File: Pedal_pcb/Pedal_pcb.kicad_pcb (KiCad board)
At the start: 2 copper layers, 40.5 x 48.5 mm, 18 parts, among them U1 TL082

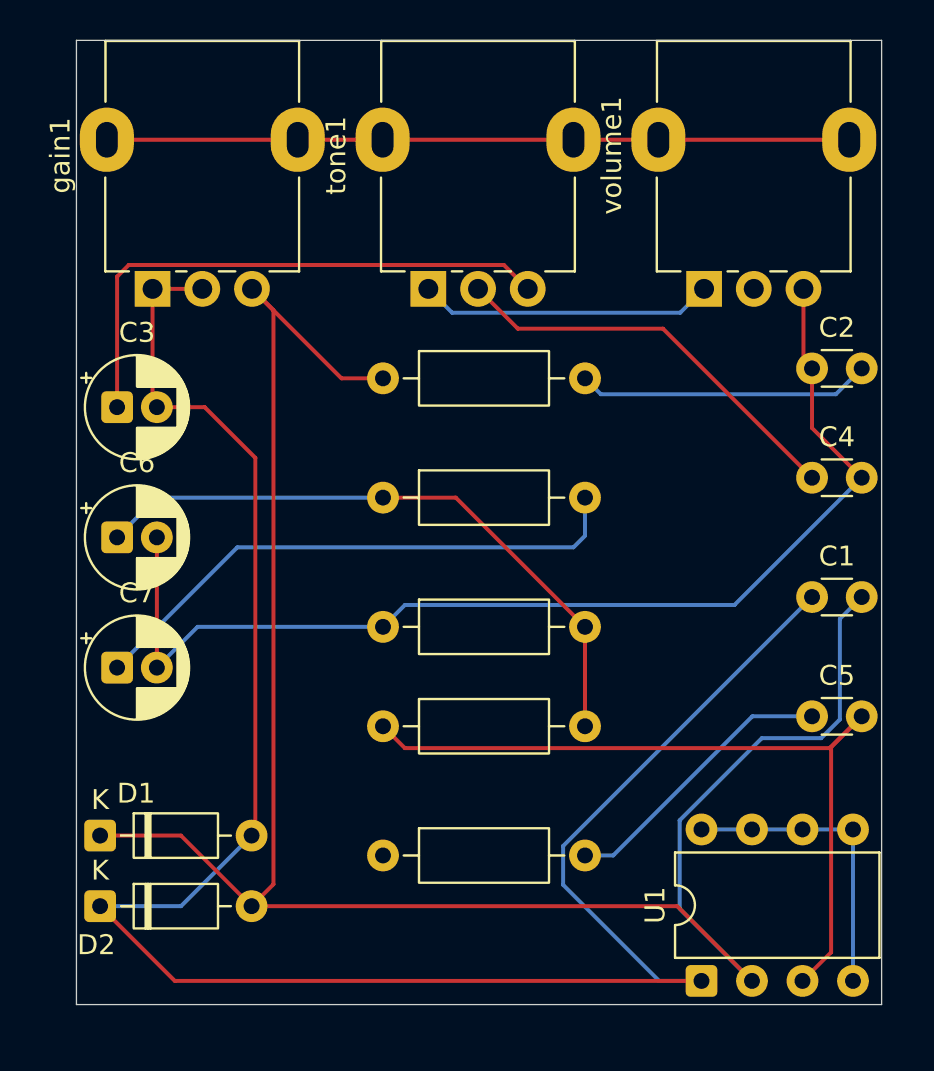
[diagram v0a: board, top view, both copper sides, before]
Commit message: better pcb design
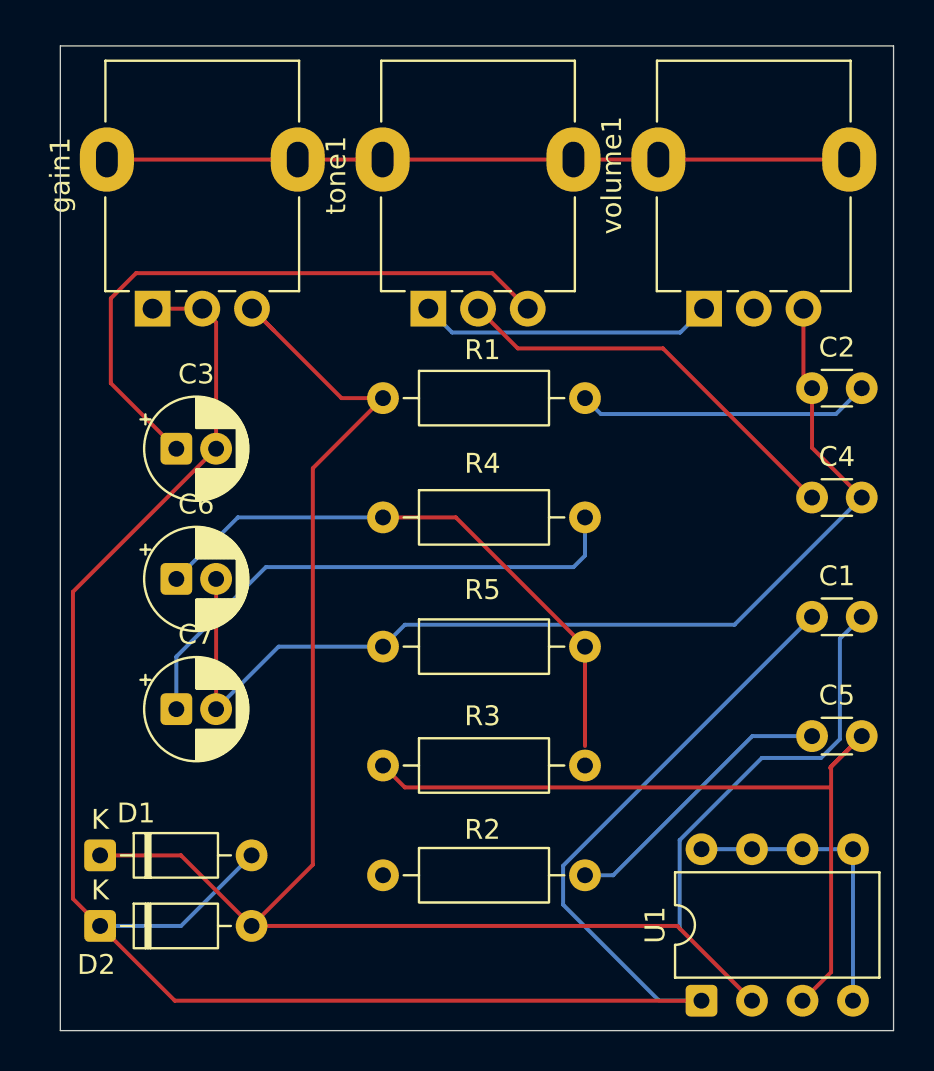
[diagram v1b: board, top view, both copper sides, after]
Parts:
- moved C6 3.64 mm to (129.0, 44.6)
- moved C7 3.64 mm to (129.0, 51.1)
- moved C3 3.64 mm to (129.0, 38.0)
- moved R3 1.98 mm to (139.4, 54.0)
- moved D2 1.00 mm to (125.2, 62.0)
- moved U1 1.00 mm to (155.4, 65.8)
- moved gain1 1.00 mm to (127.8, 31.0)
- moved tone1 1.00 mm to (141.7, 31.0)
- moved volume1 1.00 mm to (155.6, 31.0)
- moved C1 0.99 mm to (161.0, 46.5)
- moved C2 0.99 mm to (161.0, 35.0)
- moved C4 0.99 mm to (161.0, 40.5)
- moved C5 0.99 mm to (161.0, 52.5)
- moved D1 0.99 mm to (125.2, 58.5)
- moved R1 0.99 mm to (139.4, 35.5)
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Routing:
- net Net-(D1-A): track 103.2 -> 107.5 mm
- net Net-(C3-Pad1): track 28.0 -> 31.2 mm
- net GND: track 56.7 -> 54.1 mm
- net Net-(C6-Pad1): track 32.1 -> 29.5 mm
- net Net-(D1-K): track 102.6 -> 101.4 mm
- net Net-(BT1-+): track 28.2 -> 27.2 mm
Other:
- board size 40.5 x 48.5 mm -> 41.9 x 49.5 mm
- board text added: "Made in italy by italians"
- board text added: "R1"
- board text added: "R2"
- board text added: "R3"
- board text added: "R4"
- board text added: "R5"
- board text removed: "Made in italy by one italian"
